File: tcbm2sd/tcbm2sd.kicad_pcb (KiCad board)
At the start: 2 copper layers, 58.4 x 91 mm, 27 parts, among them J1 TCBM, J2 JTAG, J4 AMS1117, J5 SD CARD, J7 ALT_A6_A7, SW1 BUT_PREV, SW2 BUT_NEXT, U1 XC9572XL-VQ64, U2 Arduino Pro Mini, U3 AMS1117-3.3, U4 27C512, U5 C16_NEWSTYLE_EXP_PORT

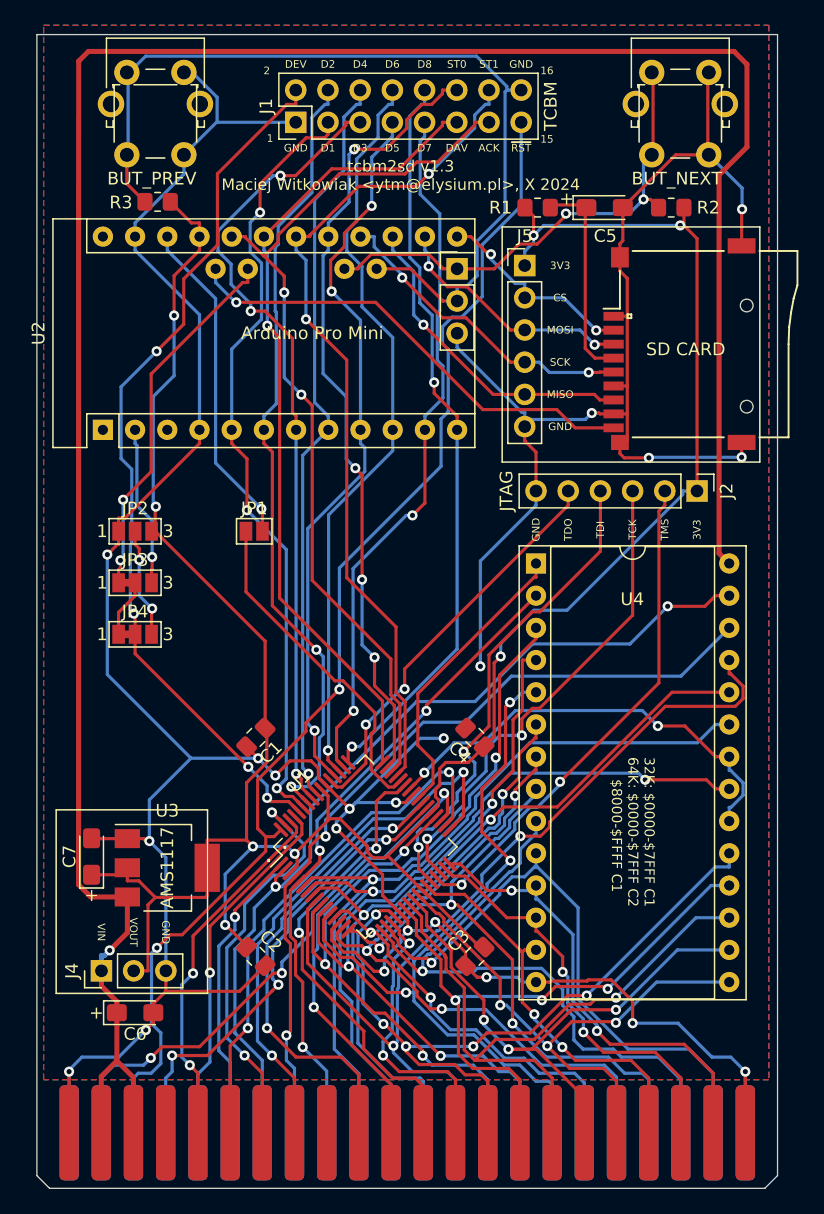
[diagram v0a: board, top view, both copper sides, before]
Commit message: Retouching
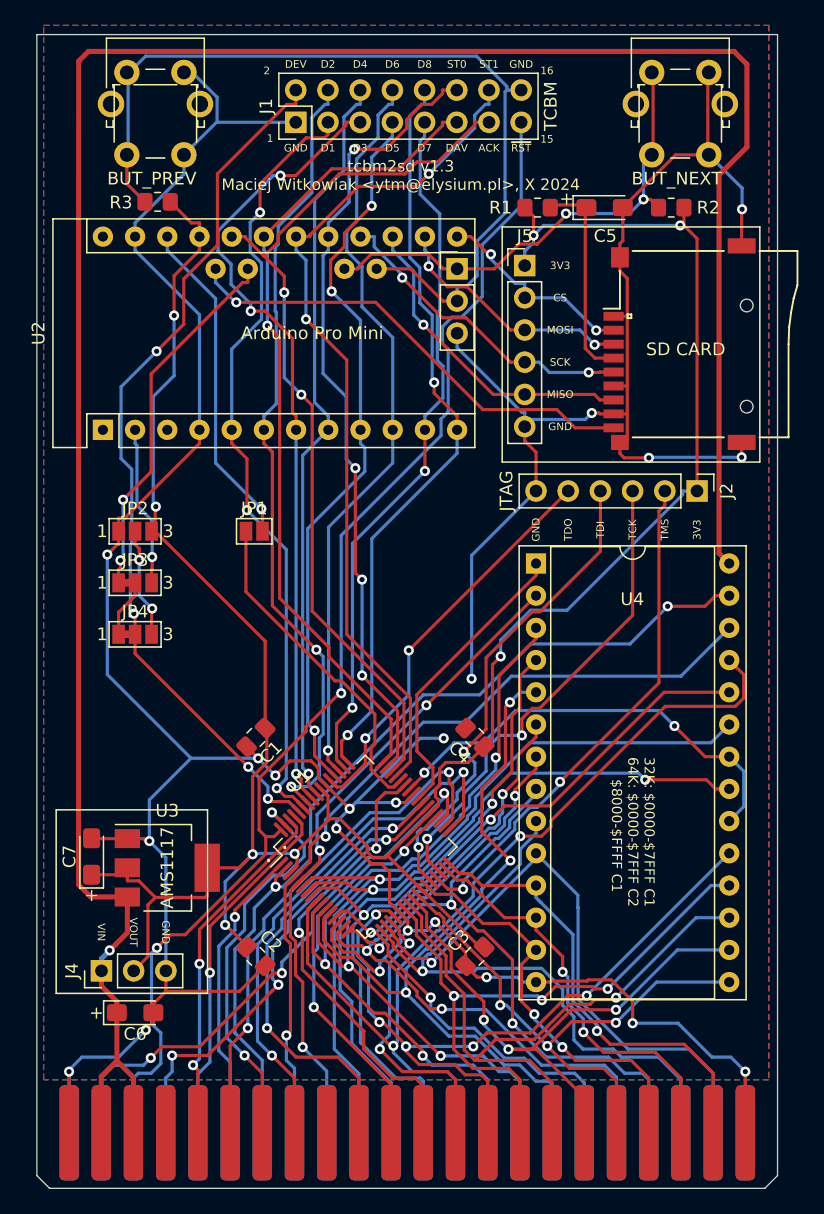
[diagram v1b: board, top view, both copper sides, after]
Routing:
- net +3V3: track 203.3 -> 200.9 mm
- net GND: track 318.5 -> 320.0 mm
- net /R/~{W}: track 29.1 -> 28.4 mm
- net /D0: track 35.9 -> 36.6 mm, vias 2 -> 1
- net /A11: track 61.7 -> 62.3 mm
- net /A6: track 59.9 -> 59.3 mm
- net /TMS: track 40.3 -> 40.8 mm
- net /DAV: track 64.4 -> 65.0 mm
- net /D7: track 58.9 -> 58.3 mm
- net /D2: track 31.7 -> 32.3 mm
